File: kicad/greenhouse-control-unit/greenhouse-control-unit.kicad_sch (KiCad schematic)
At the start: 69 parts, among them J1 Pluggable_Terminal_01x02, J10 Molex_KK-254_01x10, J10_LittleBuck1 Conn_01x01_Female, J11_LittleBuck1 Conn_01x01_Female, J12_BigBuck1 Conn_01x01_Female, J13_BigBuck1 Conn_01x01_Female, J14_LittleBuck1 Conn_01x01_Female, J15_LittleBuck1 Conn_01x01_Female, J2 Pluggable_Terminal_01x02, J3 Pluggable_Terminal_01x02, J4 Molex_KK-254_01x08, J5 Conn_01x10_Female, J6 Conn_01x10_Female, J6_BigBuck1 Conn_01x01_Female, J7 Conn_01x15_Female, J7_BigBuck1 Conn_01x01_Female, J8 Conn_01x15_Female, J9 Molex_KK-396_01x16, Q1 2N7000, Q10 IRLB8721PBF, Q11 IRLB8721PBF, Q2 2N7000, Q3 2N7000, Q4 IRLB8721PBF, Q5 IRLB8721PBF, Q6 IRLB8721PBF, Q7 IRLB8721PBF, Q8 IRLB8721PBF, Q9 IRLB8721PBF, U1 74HC595, U2 74HC595

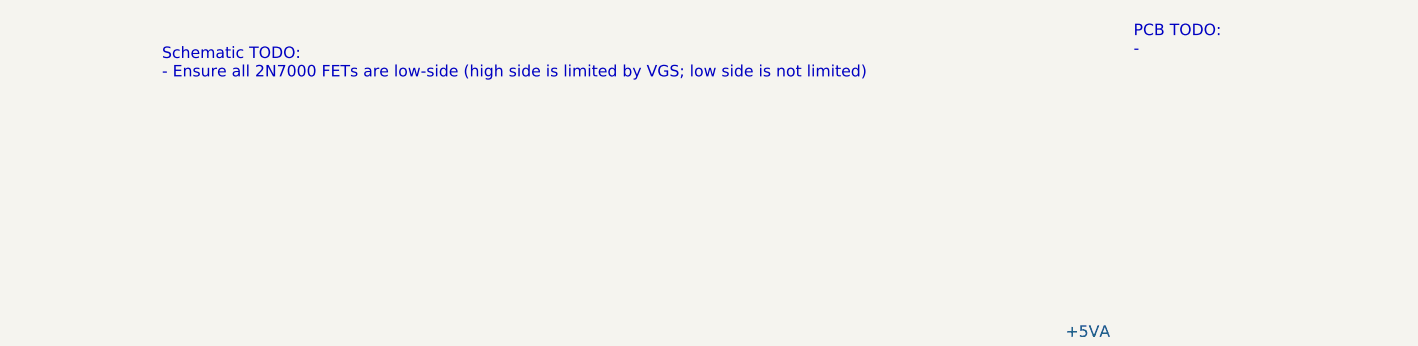
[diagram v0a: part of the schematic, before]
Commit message: Update TODO and ignore file
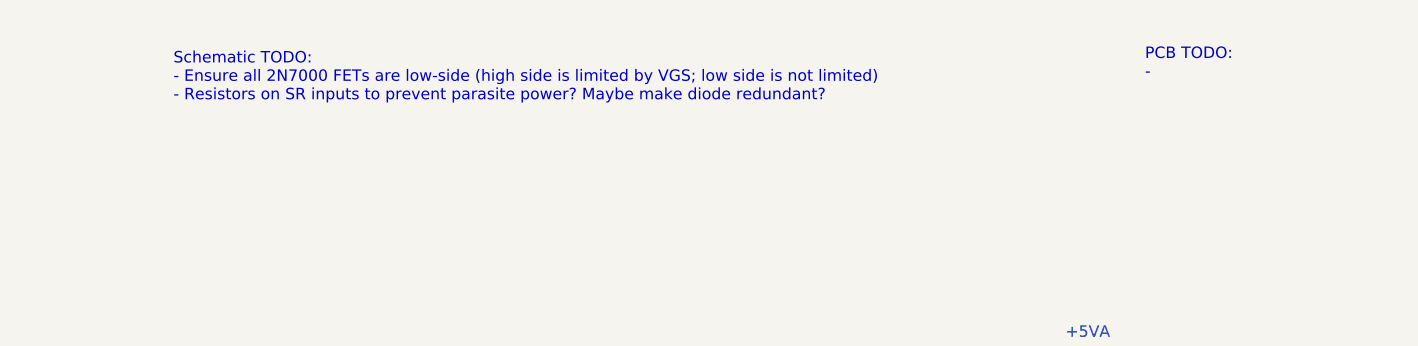
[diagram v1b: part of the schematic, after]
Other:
- note added: "Schematic TODO: - Ensure all 2N7000 FETs are low-side (high side is limited by VGS; low side is not limited) - Resistors on SR inputs to prevent parasite power? Maybe make diode redundant?"
- note removed: "Schematic TODO: - Ensure all 2N7000 FETs are low-side (high side is limited by VGS; low side is not limited)"
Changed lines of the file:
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@@
     (effects (font (size 1.27 1.27)) (justify left bottom))
   )
-  (text "PCB TODO:\n- " (at 238.76 21.59 0)
+  (text "PCB TODO:\n- " (at 240.03 24.13 0)
     (effects (font (size 1.27 1.27)) (justify left bottom))
   )
@@
     (effects (font (size 1.27 1.27)) (justify left bottom))
   )
-  (text "Schematic TODO:\n- Ensure all 2N7000 FETs are low-side (high side is limited by VGS; low side is not limited)\n"
-    (at 130.81 24.13 0)
+  (text "Schematic TODO: \n- Ensure all 2N7000 FETs are low-side (high side is limited by VGS; low side is not limited)\n- Resistors on SR inputs to prevent parasite power? Maybe make diode redundant?"
+    (at 132.08 26.67 0)
     (effects (font (size 1.27 1.27)) (justify left bottom))
   )
@@
     )
   )
-  (symbol (lib_id "power:+5V") (at 120.65 217.17 0) (unit 1)
-    (in_bom yes) (on_board yes) (fields_autoplaced)
-    (property "Reference" "#PWR07" (id 0) (at 120.65 220.98 0)
-      (effects (font (size 1.27 1.27)) hide)
-    )
-    (property "Value" "+5V" (id 1) (at 120.65 212.09 0))
-    (property "Footprint" "" (id 2) (at 120.65 217.17 0)
-      (effects (font (size 1.27 1.27)) hide)
-    )
-    (property "Datasheet" "" (id 3) (at 120.65 217.17 0)
-      (effects (font (size 1.27 1.27)) hide)
-    )
-    (pin "1")
-  )
   (symbol (lib_id "power:GND") (at 233.68 243.84 0) (unit 1)
     (in_bom yes) (on_board yes) (fields_autoplaced)
@@
     (pin "2")
   )
+  (symbol (lib_id "power:+5V") (at 120.65 217.17 0) (unit 1)
+    (in_bom yes) (on_board yes) (fields_autoplaced)
+    (property "Reference" "#PWR?" (id 0) (at 120.65 220.98 0)
+      (effects (font (size 1.27 1.27)) hide)
+    )
+    (property "Value" "+5V" (id 1) (at 120.65 212.09 0))
+    (property "Footprint" "" (id 2) (at 120.65 217.17 0)
+      (effects (font (size 1.27 1.27)) hide)
+    )
+    (property "Datasheet" "" (id 3) (at 120.65 217.17 0)
+      (effects (font (size 1.27 1.27)) hide)
+    )
+    (pin "1")
+  )
   (symbol (lib_id "power:+3V3") (at 189.23 59.69 0) (unit 1)
     (in_bom yes) (on_board yes) (fields_autoplaced)
@@
       (reference "#PWR06") (unit 1) (value "GND") (footprint "")
     )
-    (path "/270b5206-01f6-4326-bca0-f1b215f9f6ac"
-      (reference "#PWR07") (unit 1) (value "+5V") (footprint "")
-    )
     (path "/14624e4f-3e7f-43e4-90a1-bcd722e8b790"
       (reference "#PWR08") (unit 1) (value "+5V") (footprint "")
@@
       (reference "#PWR044") (unit 1) (value "+12V") (footprint "")
     )
+    (path "/b3a04bcd-a8de-4fd3-afa7-99bb35daab3f"
+      (reference "#PWR?") (unit 1) (value "+5V") (footprint "")
+    )
     (path "/e9cc145f-bccc-4781-862a-a53065926266"
